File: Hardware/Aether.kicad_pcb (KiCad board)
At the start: 2 copper layers, 67.5 x 27 mm, 78 parts, among them J1 PRGM, J2 CONN-2, J3 CONN-2, J4 CONN-2, J5 CONN-2, J6 CONN-3, J7 CONN-3, Q1 IRLML6401, U1 ANTENOVA-UB, U2 ADF7012, U3 AAT1217, U4 MCP6L02T, U5 MSP430G2553-PW28, X1 VCXO, X2 8MHz

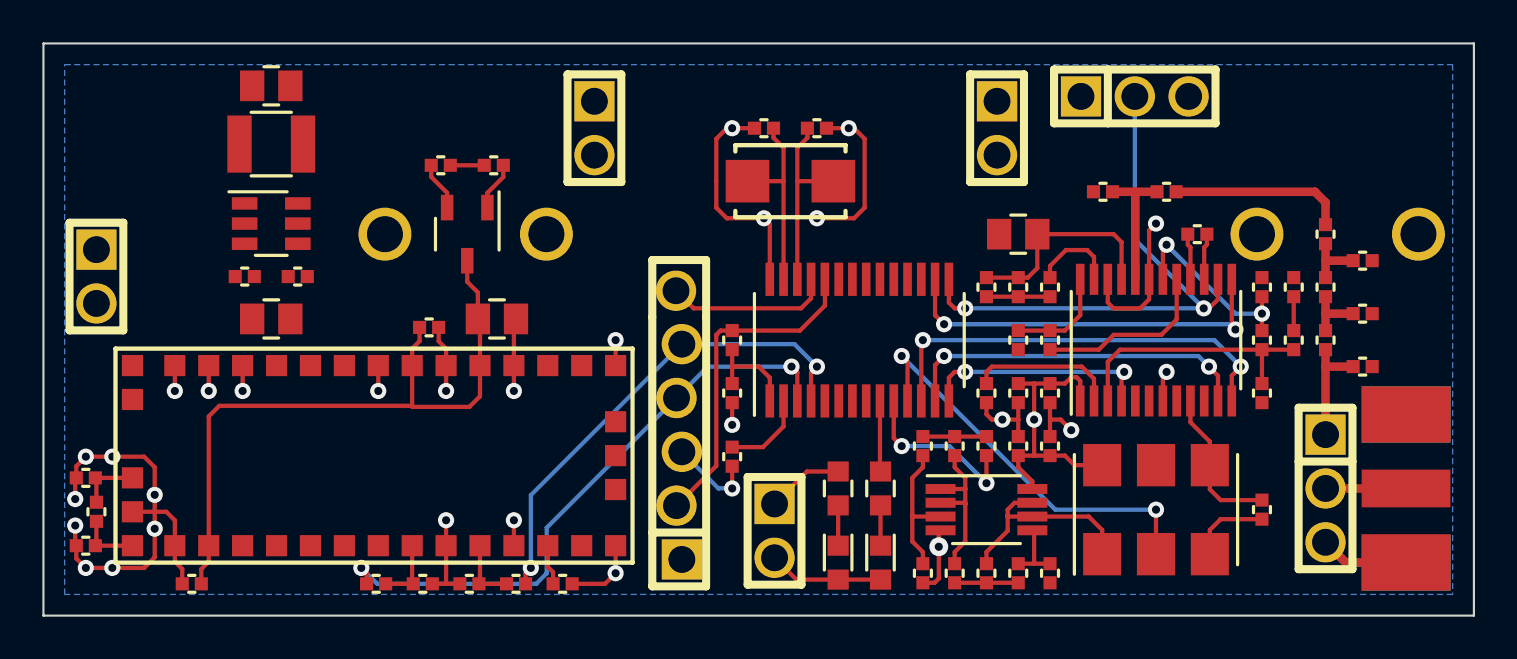
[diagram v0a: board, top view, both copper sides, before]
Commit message: Majority of layout
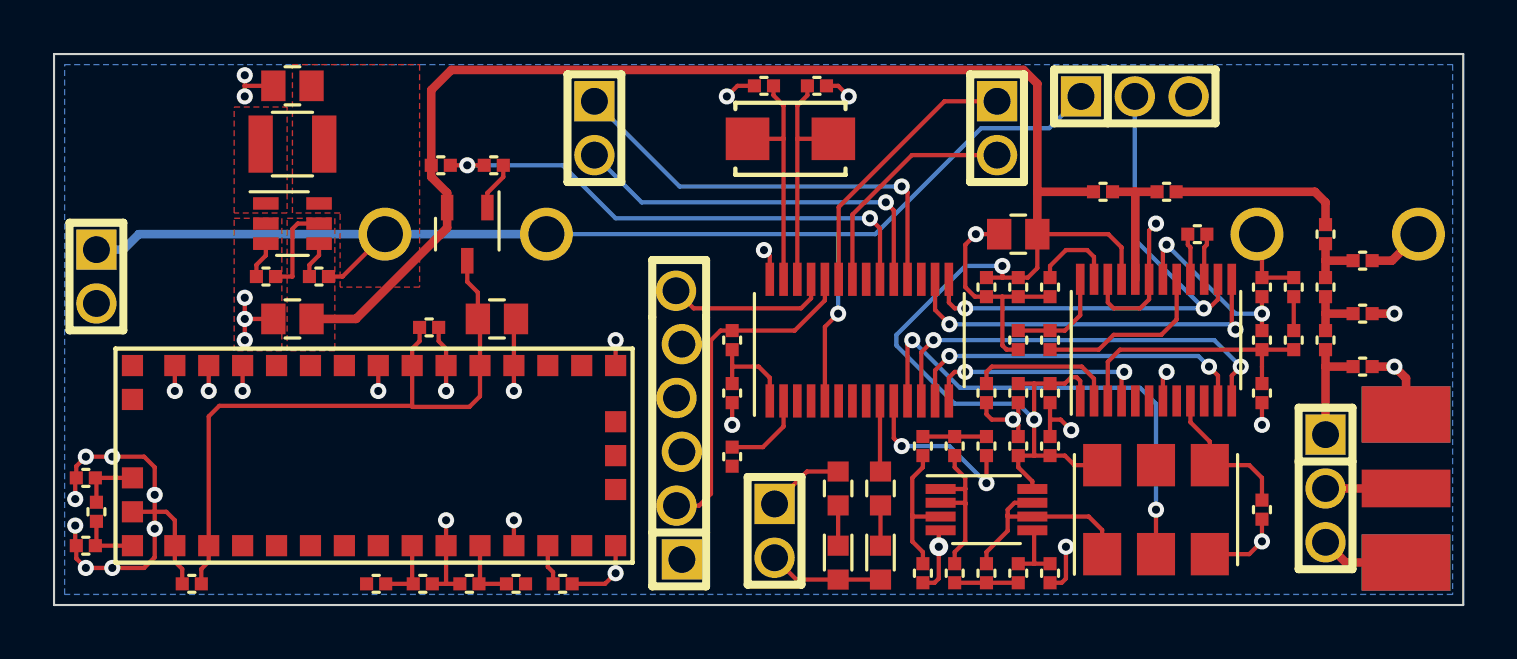
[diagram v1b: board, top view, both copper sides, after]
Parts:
- moved C31 2.00 mm to (162.0, 96.5)
- moved C33 2.00 mm to (164.5, 96.5)
- moved X2 2.00 mm to (163.2, 99.0)
- moved C24 1.00 mm to (139.8, 96.5)
- moved C28 1.00 mm to (138.5, 105.5)
- moved C29 1.00 mm to (139.8, 107.5)
- moved L8 1.00 mm to (139.8, 99.2)
- moved R9 1.00 mm to (141.0, 105.5)
- moved U3 1.00 mm to (139.8, 103.0)
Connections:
- J3 pad 1: (no net) -> /Core/E2
- J3 pad 2: (no net) -> /Core/E1
- U5 pad 18: (no net) -> /Core/E2
- U5 pad 19: (no net) -> /Core/E1
- U5 pad 20: (no net) -> /Core/GPS_En
- U5 pad 6: (no net) -> /Core/GPS_Perf
- U5 pad 7: /Core/GPS_Perf -> (no net)
- U5 pad 8: /Core/GPS_En -> (no net)
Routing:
- net +3.3V: track 36.1 -> 107.4 mm, vias 1 -> 2
- net +BATT: track 0.00 -> 61.1 mm, vias 0 -> 1
- net /Core/RX: track 28.7 -> 0.00 mm, vias 2 -> 0
- net /Core/GPS_En: track 1.60 -> 24.7 mm, vias 0 -> 2
- net /GPS/RX: track 22.9 -> 0.00 mm, vias 2 -> 0
- net /Core/E2: track 0.00 -> 20.7 mm, vias 0 -> 1
- net /Core/E1: track 0.00 -> 18.5 mm, vias 0 -> 1
- net /Core/SDA: track 0.00 -> 12.9 mm
- net /Core/SCL: track 0.00 -> 11.0 mm
- net GND: track 100.8 -> 110.5 mm, vias 28 -> 38
- net +5V: track 4.14 -> 0.00 mm, vias 1 -> 0
- net /Core/CLK_En: track 19.3 -> 22.8 mm
- net /Core/XOut: track 9.03 -> 11.0 mm
- net /Core/XIn: track 9.03 -> 11.0 mm
- net N-0000064: track 0.00 -> 1.74 mm
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- added copper zone on F.Cu, net +3.3V
- added copper zone on F.Cu, net +BATT
- added copper zone on F.Cu, net /Core/Lx
- added copper zone on F.Cu, net GND
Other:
- board size 67.5 x 27 mm -> 66.5 x 26 mm
